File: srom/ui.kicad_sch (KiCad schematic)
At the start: 7 parts, among them J301 Conn_01x10_Female, J302 Conn_01x06_Female, J303 Conn_01x03_Female, J304 Conn_01x05_Female, U301 Pico-3 UI

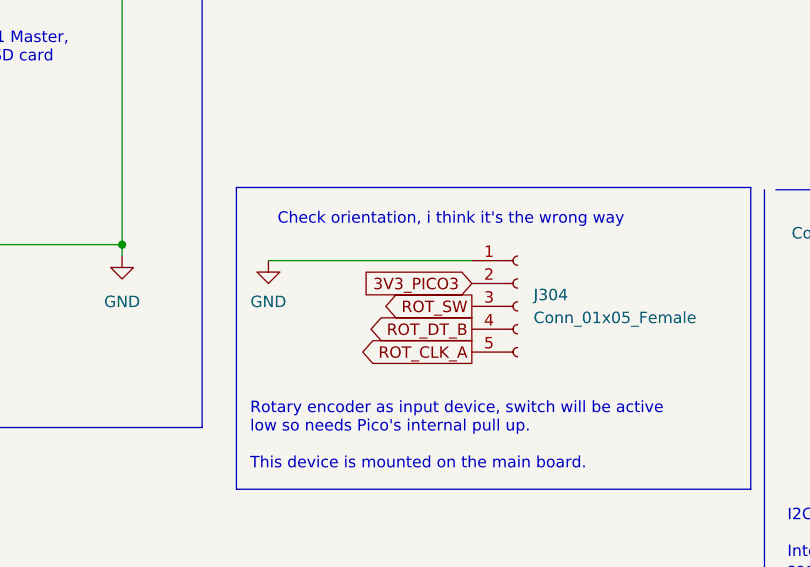
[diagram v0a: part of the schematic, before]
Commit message: more work on the new pcb, i think i have the basic layout now
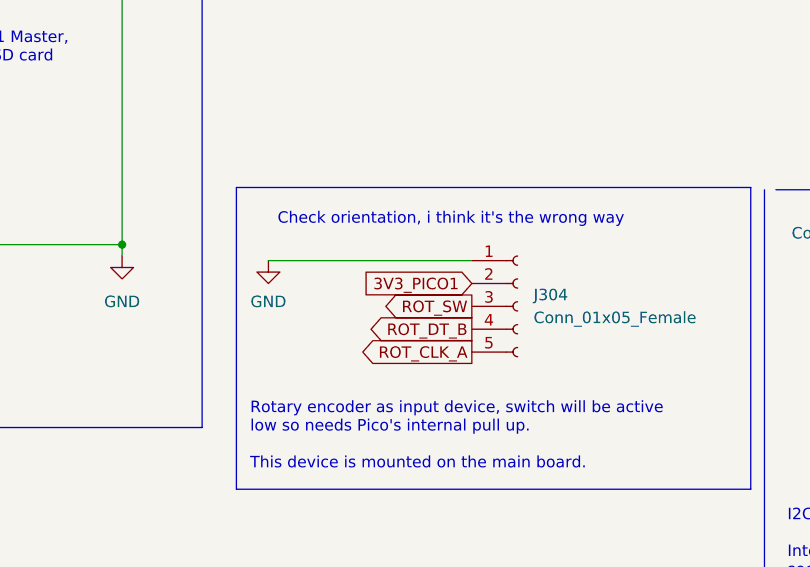
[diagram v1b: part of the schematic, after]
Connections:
- net 3V3_PICO3: no longer J304.2 (Pin_2)
- new net 3V3_PICO1: J304.2 (Pin_2)
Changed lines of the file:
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@@
     )
   )
-  (global_label "3V3_PICO3" (shape input) (at 158.242 116.078 180) (fields_autoplaced)
+  (global_label "3V3_PICO1" (shape input) (at 158.242 116.078 180) (fields_autoplaced)
     (effects (font (size 1.27 1.27)) (justify right))
     (property "Intersheet References" "${INTERSHEET_REFS}" (id 0) (at 145.6689 115.9986 0)

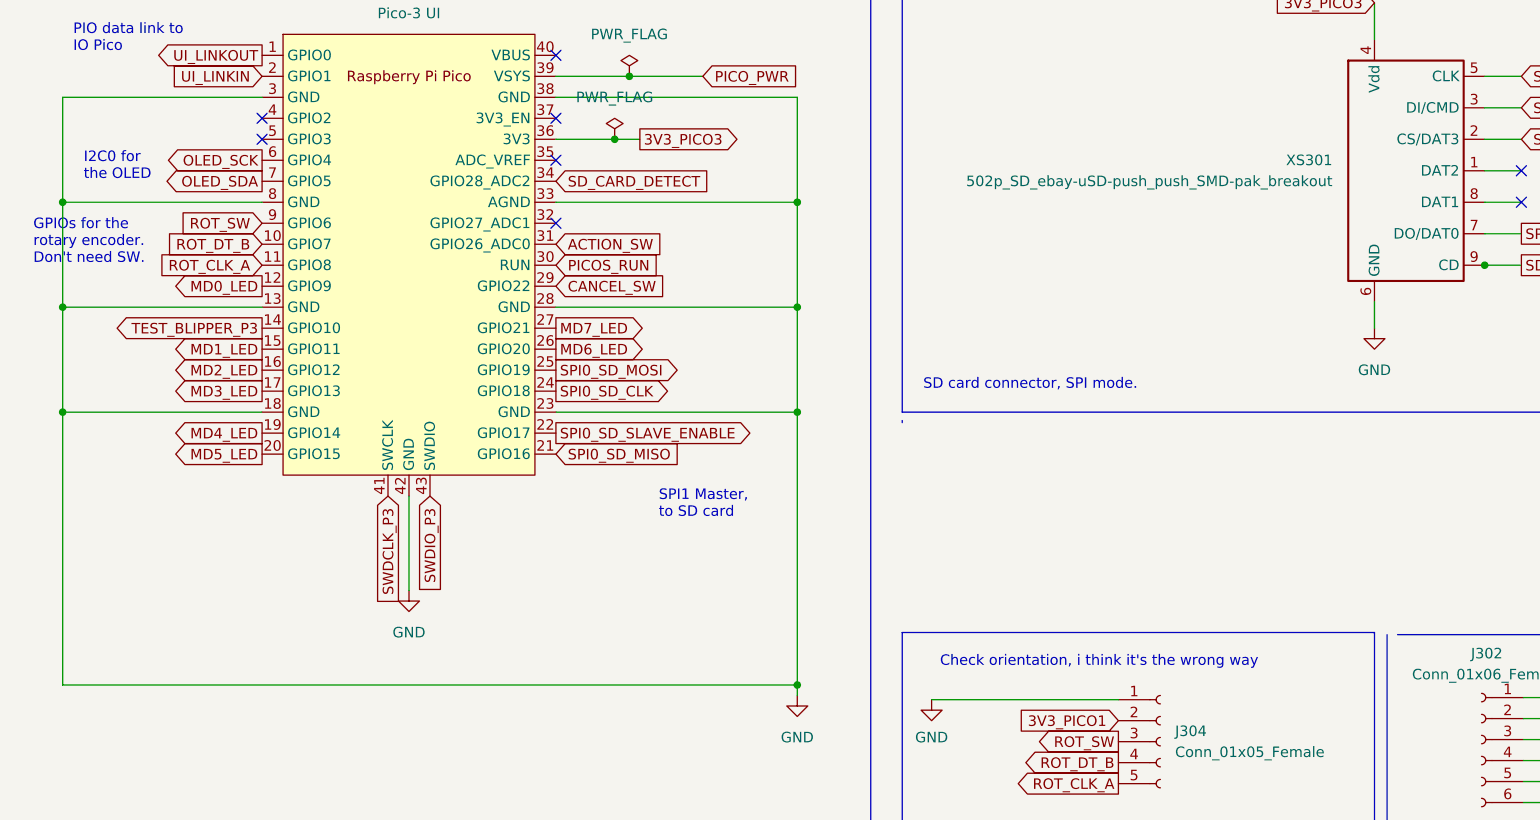
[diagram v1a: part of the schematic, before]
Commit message: final pcb? about to copy layout for daughterboard
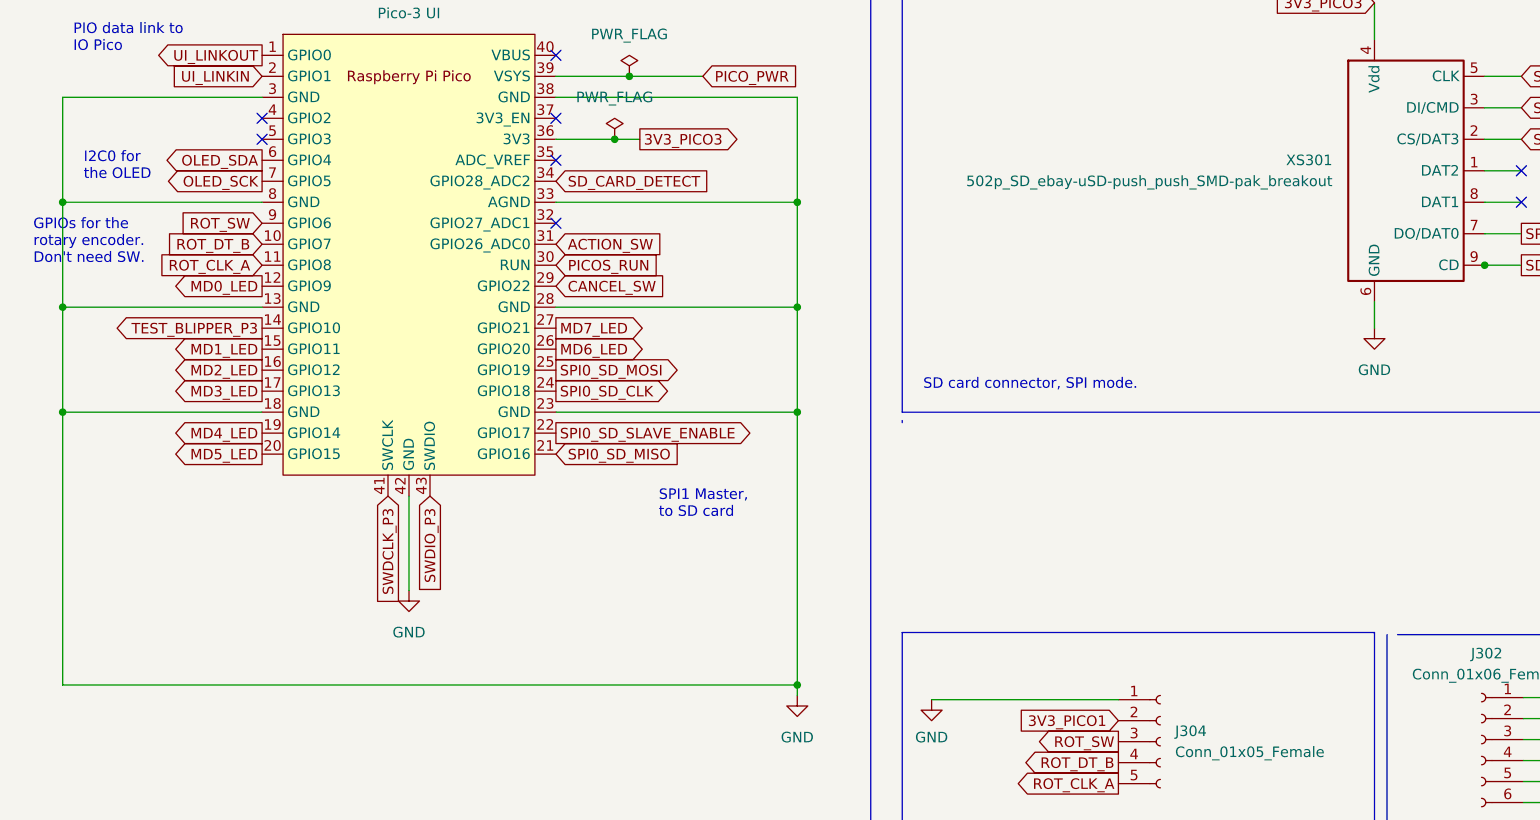
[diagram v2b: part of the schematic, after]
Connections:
- net OLED_SCK: now also U301.7 (GPIO5); no longer U301.6 (GPIO4)
- net OLED_SDA: now also U301.6 (GPIO4); no longer U301.7 (GPIO5)
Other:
- note removed: "Check orientation, i think it's the wrong way"
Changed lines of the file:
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@@
-    (effects (font (size 1.27 1.27)) (justify left bottom))
-  )
-  (text "Check orientation, i think it's the wrong way\n" (at 136.652 109.728 0)
     (effects (font (size 1.27 1.27)) (justify left bottom))
   )
@@
     )
   )
-  (global_label "OLED_SDA" (shape output) (at 54.61 50.8 180) (fields_autoplaced)
+  (global_label "OLED_SDA" (shape output) (at 54.61 48.26 180) (fields_autoplaced)
     (effects (font (size 1.27 1.27)) (justify right))
-    (property "Intersheet References" "${INTERSHEET_REFS}" (id 0) (at 42.8836 50.7206 0)
+    (property "Intersheet References" "${INTERSHEET_REFS}" (id 0) (at 42.8836 48.1806 0)
       (effects (font (size 1.27 1.27)) (justify right) hide)
     )
@@
     )
   )
-  (global_label "OLED_SCK" (shape output) (at 54.61 48.26 180) (fields_autoplaced)
+  (global_label "OLED_SCK" (shape output) (at 54.61 50.8 180) (fields_autoplaced)
     (effects (font (size 1.27 1.27)) (justify right))
-    (property "Intersheet References" "${INTERSHEET_REFS}" (id 0) (at 42.7021 48.1806 0)
+    (property "Intersheet References" "${INTERSHEET_REFS}" (id 0) (at 42.7021 50.7206 0)
       (effects (font (size 1.27 1.27)) (justify right) hide)
     )
